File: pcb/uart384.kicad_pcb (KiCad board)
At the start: 2 copper layers, 56.6 x 23.5 mm, 32 parts, among them IC1 ICE40LP384-SG32, J1 USB_A, J2 TC2050, J3 Conn_02x06_Odd_Even, SW1 SW_Push, U1 CP2102-QFN28, U2 AT25DF256-XMHN-T, U3 MIC5365-1.2YC5, Y1 XO32

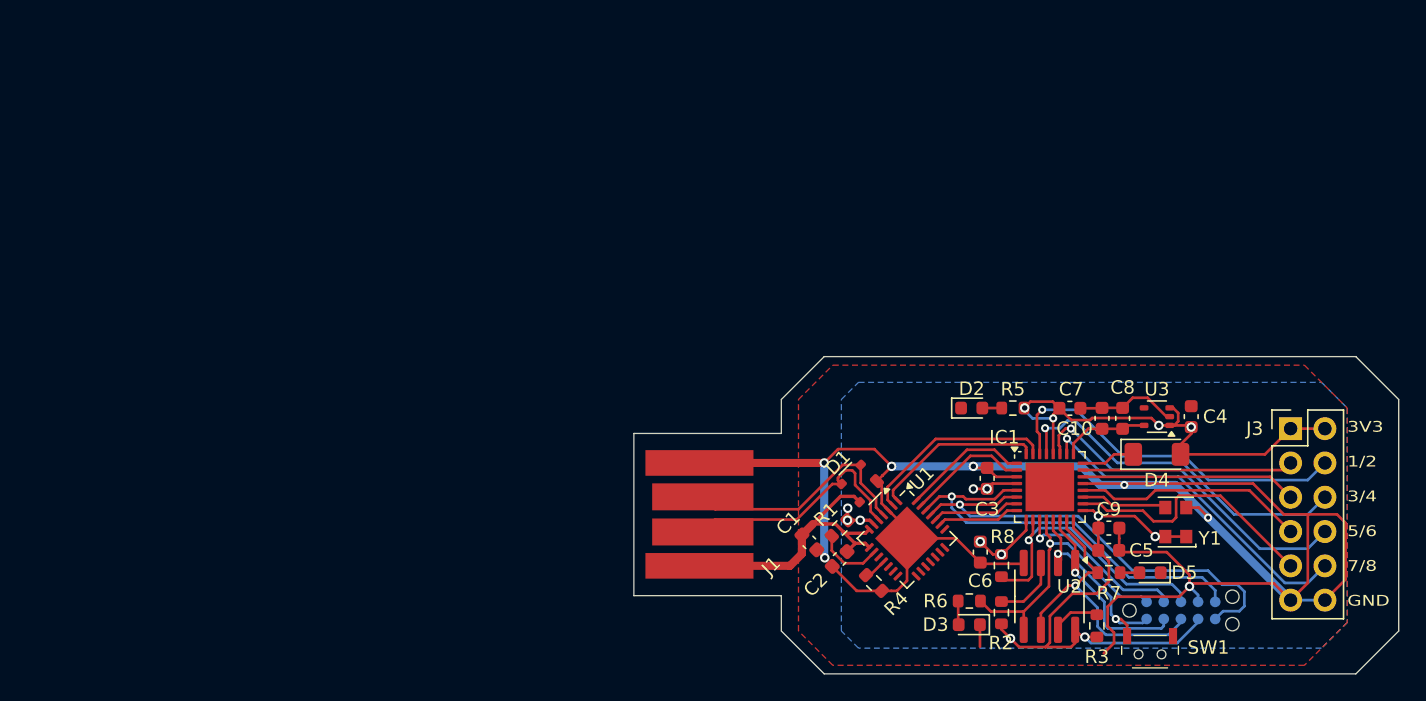
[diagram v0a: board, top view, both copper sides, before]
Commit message: release PCB v1.0: setup production files, docs
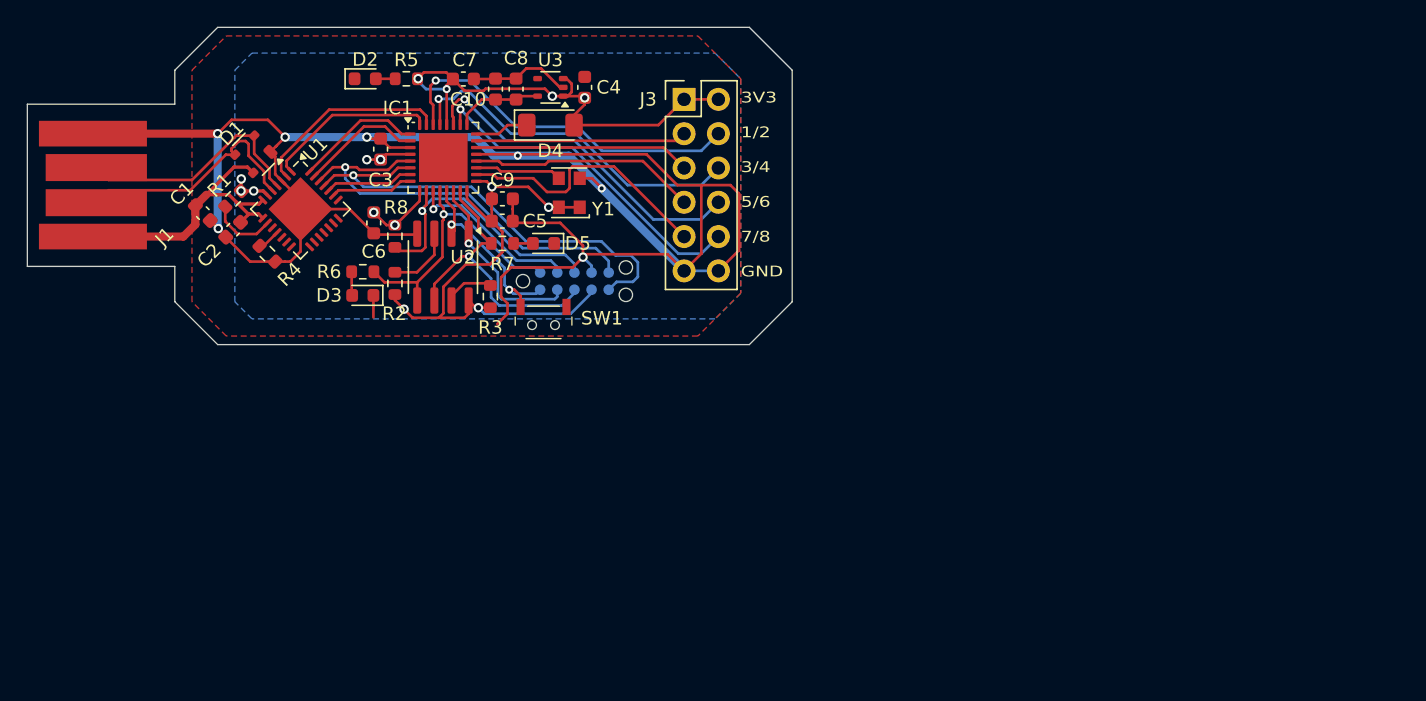
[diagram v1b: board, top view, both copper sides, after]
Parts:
- moved C10 51.1 mm to (110.9, 69.1)
- moved C5 51.1 mm to (111.4, 78.9)
- moved C6 51.1 mm to (101.9, 79.0)
- moved C8 51.1 mm to (112.4, 69.1)
- moved J3 51.1 mm to (124.9, 69.8)
- moved R3 51.1 mm to (110.5, 84.5)
- moved U1 51.1 mm to (96.5, 78.0)
- moved C1 51.1 mm to (89.2, 78.3)
- moved C2 51.1 mm to (91.5, 79.5)
- moved C3 51.1 mm to (102.4, 73.5)
- moved C4 51.1 mm to (117.5, 69.0)
- moved D1 51.1 mm to (93.0, 73.9)
- moved D2 51.1 mm to (101.3, 68.3)
- moved D3 51.1 mm to (101.1, 84.4)
- moved D4 51.1 mm to (115.0, 71.8)
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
